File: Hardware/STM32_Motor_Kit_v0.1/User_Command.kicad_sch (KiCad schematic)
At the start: 6 parts, among them SW3 Push_Button_SMD_4P

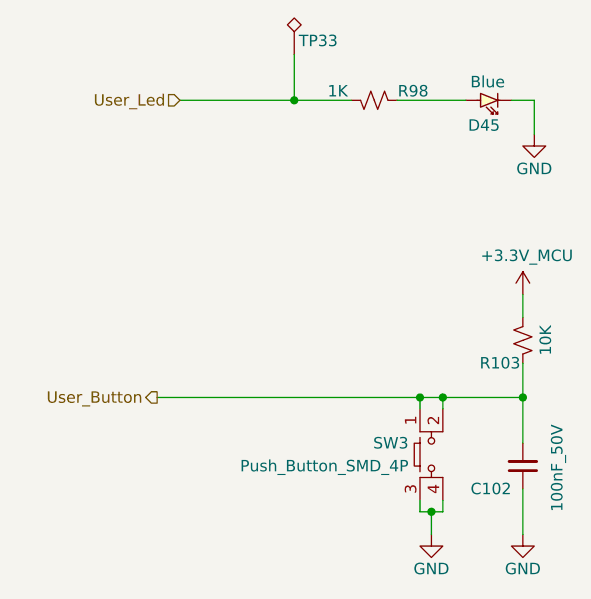
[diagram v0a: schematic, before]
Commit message: 12.01.2025
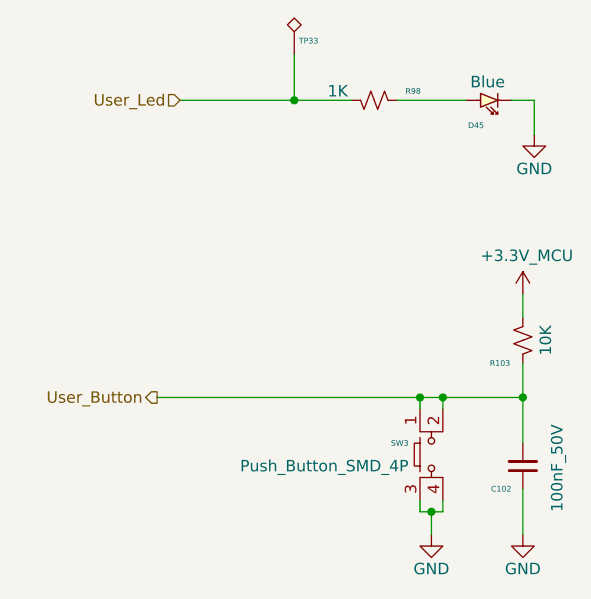
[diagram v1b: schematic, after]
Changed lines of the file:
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@@
 			(effects
 				(font
-					(size 1.27 1.27)
+					(face "Arial")
+					(size 0.635 0.635)
 				)
 				(hide yes)
@@
 			(effects
 				(font
-					(size 1.27 1.27)
+					(face "Arial")
+					(size 0.635 0.635)
 				)
 				(justify left)
@@
 			(effects
 				(font
-					(size 1.27 1.27)
+					(face "Arial")
+					(size 0.635 0.635)
 				)
 				(hide yes)
@@
 			(effects
 				(font
-					(size 1.27 1.27)
+					(face "Arial")
+					(size 0.635 0.635)
 				)
 				(hide yes)
@@
 			(effects
 				(font
-					(size 1.27 1.27)
+					(face "Arial")
+					(size 0.635 0.635)
 				)
 				(justify right)
@@
 			(effects
 				(font
-					(size 1.27 1.27)
+					(face "Arial")
+					(size 0.635 0.635)
 				)
 			)
@@
 			(effects
 				(font
-					(size 1.27 1.27)
+					(face "Arial")
+					(size 0.635 0.635)
 				)
 				(justify left)
@@
 			(effects
 				(font
-					(size 1.27 1.27)
+					(face "Arial")
+					(size 0.635 0.635)
 				)
 				(hide yes)
@@
 			(effects
 				(font
-					(size 1.27 1.27)
+					(face "Arial")
+					(size 0.635 0.635)
 				)
 				(justify right)
@@
 			(effects
 				(font
-					(size 1.27 1.27)
-				)
-			)
+					(face "Arial")
+					(size 0.635 0.635)
+				)
+			)
